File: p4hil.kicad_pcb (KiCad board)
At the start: 4 copper layers, 81.3 x 50.8 mm, 216 parts, among them J1 Conn_02x02_Odd_Even, J10 Conn_01x20, J11 Conn_01x20, J12 Conn_01x20, J13 USB_A_Stacked, J14 Conn_01x04, J15 Conn_01x20, J16 Conn_01x04, J17 Barrel_Jack_Switch, J18 Conn_02x05_Odd_Even, J19 HR871150C, J2 Conn_01x08, J3 USB_C_Receptacle_USB2.0_16P, J4 Conn_01x10, J5 Conn_01x20, J6 Conn_01x20, J7 Conn_01x20, J8 Conn_01x02, J9 Conn_01x06, SW1 SW_Push, SW2 SW_Push, U1 W25Q128JVS, U10 TLV62569DBV, U11 MT9700_SY6280, U3 TLV62569DBV, U4 IPGRI, U6 INA219AxD, U7 CH334F, U8 MT9700_SY6280, U9 MT9700_SY6280, Y1 40MHz(+-10 ppm) C501798, Y2 25Mhz 12pf, Y3 12MHz

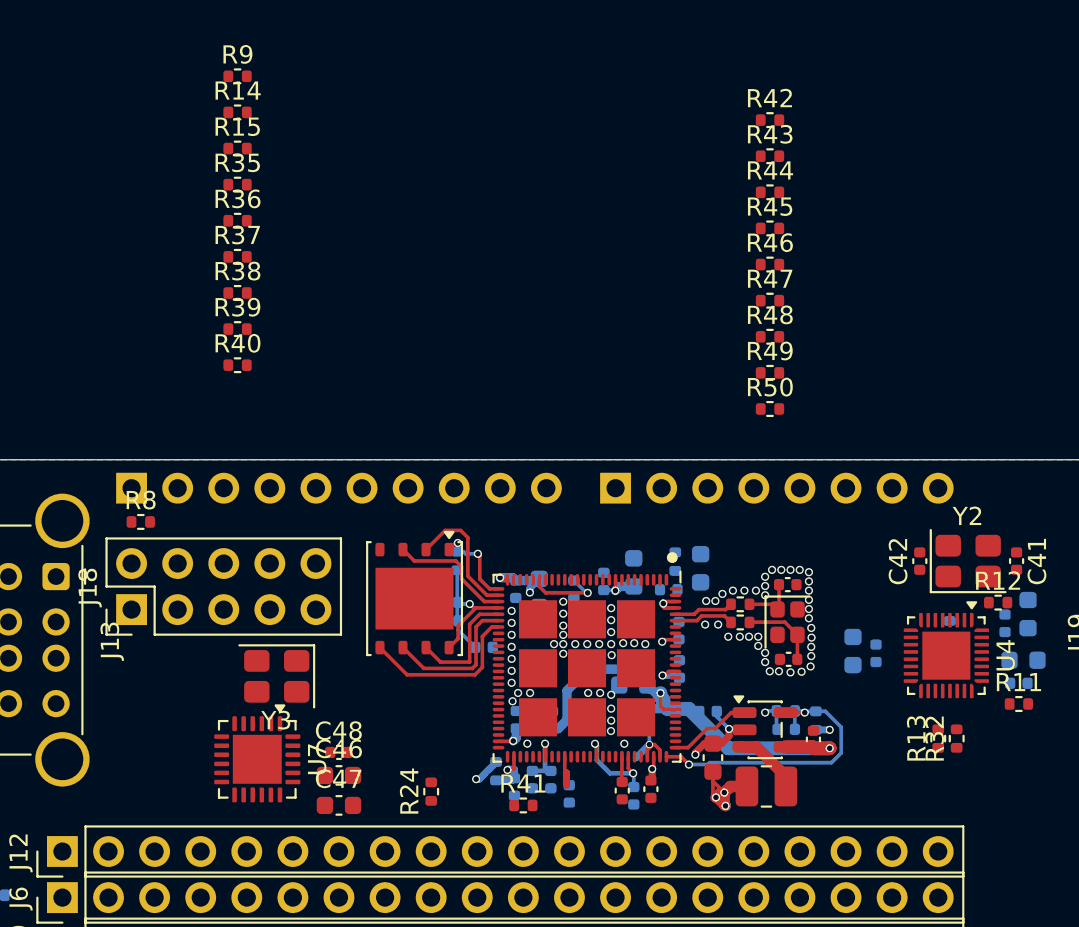
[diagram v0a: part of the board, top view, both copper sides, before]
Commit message: Drop T20'
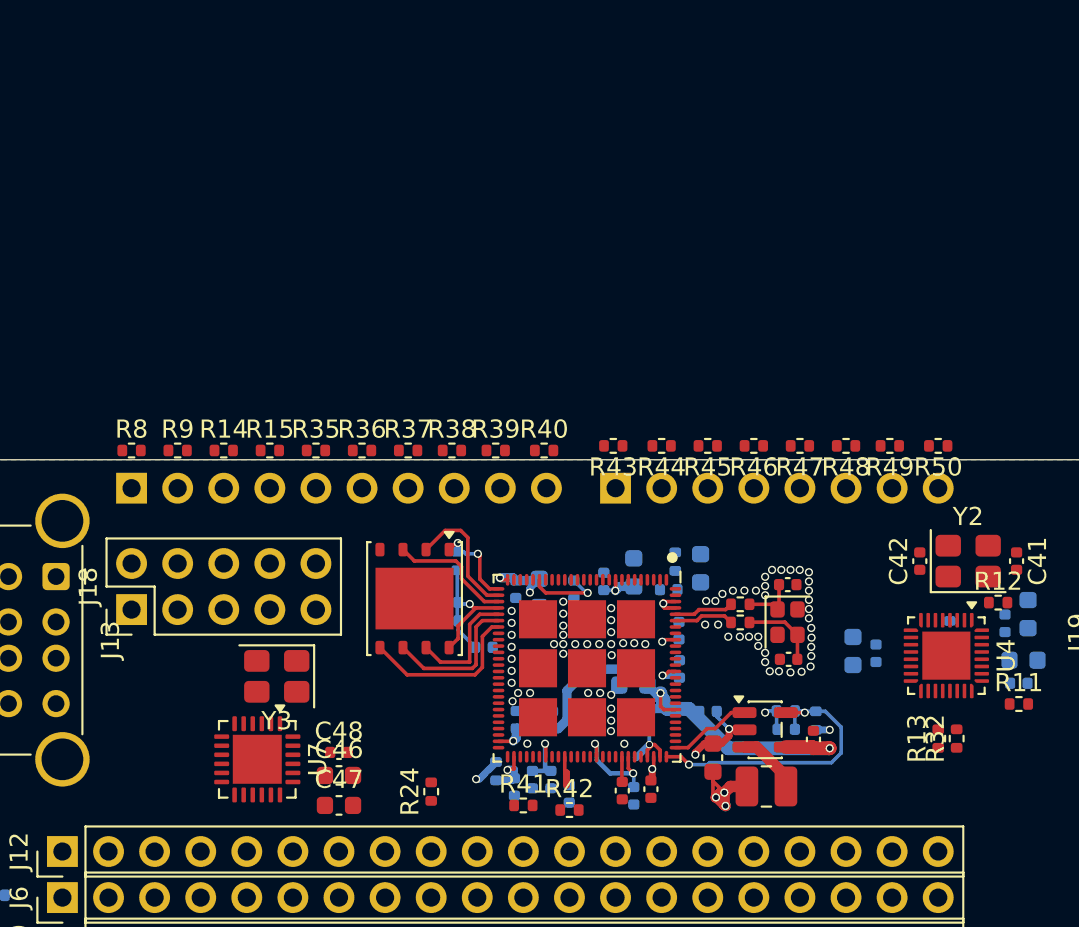
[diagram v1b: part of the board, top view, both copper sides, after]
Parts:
- moved R42 39.6 mm to (139.7, 92.7)
- moved R9 20.9 mm to (118.1, 72.9)
- moved R14 18.6 mm to (120.7, 72.9)
- moved R43 18.1 mm to (142.1, 72.6), turned to 180 degrees
- moved R40 17.5 mm to (138.3, 72.9)
- moved R15 16.7 mm to (123.2, 72.9)
- moved R39 15.7 mm to (135.6, 72.9)
- moved R35 15.3 mm to (125.7, 72.9)
- moved R44 15.2 mm to (144.8, 72.6), turned to 180 degrees
- moved R38 14.7 mm to (133.2, 72.9)
- moved R36 14.4 mm to (128.3, 72.9)
- moved R37 14.2 mm to (130.8, 72.9)
- moved R45 12.5 mm to (147.3, 72.6), turned to 180 degrees
- moved R46 10.0 mm to (149.9, 72.6), turned to 180 degrees
- moved R50 9.49 mm to (160.0, 72.6), turned to 180 degrees
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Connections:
- net /DeviceUnderTest/B1 renamed /B1
- net /DeviceUnderTest/B10 renamed /B10
- net /DeviceUnderTest/B11 renamed /B11
- net /DeviceUnderTest/B12 renamed /B12
- net /DeviceUnderTest/B13 renamed /B13
- net /DeviceUnderTest/B14 renamed /B14
- net /DeviceUnderTest/B15 renamed /B15
- net /DeviceUnderTest/B16 renamed /B16
- net /DeviceUnderTest/B17 renamed /B17
- net /DeviceUnderTest/B18 renamed /B18
- net /DeviceUnderTest/B19 renamed /B19
- net /DeviceUnderTest/B2 renamed /B2
- net /DeviceUnderTest/B20 renamed /B20
- net /DeviceUnderTest/B3 renamed /B3
- net /DeviceUnderTest/B4 renamed /B4
- net /DeviceUnderTest/B5 renamed /B5
- net /DeviceUnderTest/B6 renamed /B6
- net /DeviceUnderTest/B7 renamed /B7
- net /DeviceUnderTest/B8 renamed /B8
- net /DeviceUnderTest/B9 renamed /B9
- J10 pad 1: /DeviceUnderTest/T1 -> /DeviceUnderTest/T1i
- J10 pad 10: /DeviceUnderTest/T10 -> /DeviceUnderTest/T10i
- J10 pad 11: /DeviceUnderTest/ARDUINO_IOREF -> /DeviceUnderTest/T11i
- J10 pad 12: /DeviceUnderTest/ARDUINO_RESET -> /DeviceUnderTest/T12i
- J10 pad 13: /DeviceUnderTest/T13 -> /DeviceUnderTest/T13i
- J10 pad 14: /DeviceUnderTest/T14 -> /DeviceUnderTest/T14i
- J10 pad 15: /DeviceUnderTest/T15 -> /DeviceUnderTest/T15i
- J10 pad 16: /DeviceUnderTest/T16 -> /DeviceUnderTest/T16i
- J10 pad 17: /DeviceUnderTest/T17 -> /DeviceUnderTest/T17i
- J10 pad 18: /DeviceUnderTest/T18 -> /DeviceUnderTest/T18i
- J10 pad 19: /DeviceUnderTest/T19 -> /DeviceUnderTest/T19i
- J10 pad 2: /DeviceUnderTest/T2 -> /DeviceUnderTest/T2i
- J10 pad 20: /DeviceUnderTest/T20 -> /DeviceUnderTest/T20i
- J10 pad 3: /DeviceUnderTest/T3 -> /DeviceUnderTest/T3i
- J10 pad 4: /DeviceUnderTest/T4 -> /DeviceUnderTest/T4i
- J10 pad 5: /DeviceUnderTest/T5 -> /DeviceUnderTest/T5i
- J10 pad 6: /DeviceUnderTest/T6 -> /DeviceUnderTest/T6i
- J10 pad 7: /DeviceUnderTest/T7 -> /DeviceUnderTest/T7i
- J10 pad 8: /DeviceUnderTest/T8 -> /DeviceUnderTest/T8i
- J10 pad 9: /DeviceUnderTest/T9 -> /DeviceUnderTest/T9i
- J11 pad 1: /DeviceUnderTest/T1 -> /DeviceUnderTest/T1i
- J11 pad 10: /DeviceUnderTest/T10 -> /DeviceUnderTest/T10i
- J11 pad 11: /DeviceUnderTest/ARDUINO_IOREF -> /DeviceUnderTest/T11i
- J11 pad 12: /DeviceUnderTest/ARDUINO_RESET -> /DeviceUnderTest/T12i
- J11 pad 13: /DeviceUnderTest/T13 -> /DeviceUnderTest/T13i
- J11 pad 14: /DeviceUnderTest/T14 -> /DeviceUnderTest/T14i
- J11 pad 15: /DeviceUnderTest/T15 -> /DeviceUnderTest/T15i
- J11 pad 16: /DeviceUnderTest/T16 -> /DeviceUnderTest/T16i
- J11 pad 17: /DeviceUnderTest/T17 -> /DeviceUnderTest/T17i
- J11 pad 18: /DeviceUnderTest/T18 -> /DeviceUnderTest/T18i
- J11 pad 19: /DeviceUnderTest/T19 -> /DeviceUnderTest/T19i
- J11 pad 2: /DeviceUnderTest/T2 -> /DeviceUnderTest/T2i
- J11 pad 20: /DeviceUnderTest/T20 -> /DeviceUnderTest/T20i
- J11 pad 3: /DeviceUnderTest/T3 -> /DeviceUnderTest/T3i
- J11 pad 4: /DeviceUnderTest/T4 -> /DeviceUnderTest/T4i
- J11 pad 5: /DeviceUnderTest/T5 -> /DeviceUnderTest/T5i
- J11 pad 6: /DeviceUnderTest/T6 -> /DeviceUnderTest/T6i
- J11 pad 7: /DeviceUnderTest/T7 -> /DeviceUnderTest/T7i
- J11 pad 8: /DeviceUnderTest/T8 -> /DeviceUnderTest/T8i
- J11 pad 9: /DeviceUnderTest/T9 -> /DeviceUnderTest/T9i
- J12 pad 1: /DeviceUnderTest/T1 -> /DeviceUnderTest/T1i
- J12 pad 10: /DeviceUnderTest/T10 -> /DeviceUnderTest/T10i
- J12 pad 11: /DeviceUnderTest/ARDUINO_IOREF -> /DeviceUnderTest/T11i
- J12 pad 12: /DeviceUnderTest/ARDUINO_RESET -> /DeviceUnderTest/T12i
- J12 pad 13: /DeviceUnderTest/T13 -> /DeviceUnderTest/T13i
- J12 pad 14: /DeviceUnderTest/T14 -> /DeviceUnderTest/T14i
- J12 pad 15: /DeviceUnderTest/T15 -> /DeviceUnderTest/T15i
- J12 pad 16: /DeviceUnderTest/T16 -> /DeviceUnderTest/T16i
- J12 pad 17: /DeviceUnderTest/T17 -> /DeviceUnderTest/T17i
- J12 pad 18: /DeviceUnderTest/T18 -> /DeviceUnderTest/T18i
- J12 pad 19: /DeviceUnderTest/T19 -> /DeviceUnderTest/T19i
- J12 pad 2: /DeviceUnderTest/T2 -> /DeviceUnderTest/T2i
- J12 pad 20: /DeviceUnderTest/T20 -> /DeviceUnderTest/T20i
- J12 pad 3: /DeviceUnderTest/T3 -> /DeviceUnderTest/T3i
- J12 pad 4: /DeviceUnderTest/T4 -> /DeviceUnderTest/T4i
- J12 pad 5: /DeviceUnderTest/T5 -> /DeviceUnderTest/T5i
- J12 pad 6: /DeviceUnderTest/T6 -> /DeviceUnderTest/T6i
- J12 pad 7: /DeviceUnderTest/T7 -> /DeviceUnderTest/T7i
- J12 pad 8: /DeviceUnderTest/T8 -> /DeviceUnderTest/T8i
- J12 pad 9: /DeviceUnderTest/T9 -> /DeviceUnderTest/T9i
- J15 pad 1: /DeviceUnderTest/T1 -> /DeviceUnderTest/T1i
- J15 pad 10: /DeviceUnderTest/T10 -> /DeviceUnderTest/T10i
- J15 pad 11: /DeviceUnderTest/ARDUINO_IOREF -> /DeviceUnderTest/T11i
- J15 pad 12: /DeviceUnderTest/ARDUINO_RESET -> /DeviceUnderTest/T12i
- J15 pad 13: /DeviceUnderTest/T13 -> /DeviceUnderTest/T13i
- J15 pad 14: /DeviceUnderTest/T14 -> /DeviceUnderTest/T14i
- J15 pad 15: /DeviceUnderTest/T15 -> /DeviceUnderTest/T15i
- J15 pad 16: /DeviceUnderTest/T16 -> /DeviceUnderTest/T16i
- J15 pad 17: /DeviceUnderTest/T17 -> /DeviceUnderTest/T17i
- J15 pad 18: /DeviceUnderTest/T18 -> /DeviceUnderTest/T18i
- J15 pad 19: /DeviceUnderTest/T19 -> /DeviceUnderTest/T19i
- J15 pad 2: /DeviceUnderTest/T2 -> /DeviceUnderTest/T2i
- J15 pad 20: /DeviceUnderTest/T20 -> /DeviceUnderTest/T20i
- J15 pad 3: /DeviceUnderTest/T3 -> /DeviceUnderTest/T3i
- J15 pad 4: /DeviceUnderTest/T4 -> /DeviceUnderTest/T4i
- J15 pad 5: /DeviceUnderTest/T5 -> /DeviceUnderTest/T5i
- J15 pad 6: /DeviceUnderTest/T6 -> /DeviceUnderTest/T6i
- J15 pad 7: /DeviceUnderTest/T7 -> /DeviceUnderTest/T7i
- J15 pad 8: /DeviceUnderTest/T8 -> /DeviceUnderTest/T8i
- J15 pad 9: /DeviceUnderTest/T9 -> /DeviceUnderTest/T9i
- J2 pad 1: /DeviceUnderTest/T13 -> /DeviceUnderTest/T13i
- J2 pad 2: /DeviceUnderTest/T14 -> /DeviceUnderTest/T14i
- J2 pad 3: /DeviceUnderTest/T15 -> /DeviceUnderTest/T15i
- J2 pad 4: /DeviceUnderTest/T16 -> /DeviceUnderTest/T16i
- J2 pad 5: /DeviceUnderTest/T17 -> /DeviceUnderTest/T17i
- J2 pad 6: /DeviceUnderTest/T18 -> /DeviceUnderTest/T18i
- J2 pad 7: /DeviceUnderTest/T19 -> /DeviceUnderTest/T19i
- J2 pad 8: /DeviceUnderTest/T20 -> /DeviceUnderTest/T20i
- J4 pad 1: /DeviceUnderTest/T1 -> /DeviceUnderTest/T1i
- J4 pad 10: /DeviceUnderTest/T10 -> /DeviceUnderTest/T10i
- J4 pad 2: /DeviceUnderTest/T2 -> /DeviceUnderTest/T2i
- J4 pad 3: /DeviceUnderTest/T3 -> /DeviceUnderTest/T3i
- J4 pad 4: /DeviceUnderTest/T4 -> /DeviceUnderTest/T4i
- J4 pad 5: /DeviceUnderTest/T5 -> /DeviceUnderTest/T5i
- J4 pad 6: /DeviceUnderTest/T6 -> /DeviceUnderTest/T6i
- J4 pad 7: /DeviceUnderTest/T7 -> /DeviceUnderTest/T7i
- J4 pad 8: /DeviceUnderTest/T8 -> /DeviceUnderTest/T8i
- J4 pad 9: /DeviceUnderTest/T9 -> /DeviceUnderTest/T9i
- J6 pad 1: /DeviceUnderTest/T1 -> /DeviceUnderTest/T1i
- J6 pad 10: /DeviceUnderTest/T10 -> /DeviceUnderTest/T10i
- J6 pad 11: /DeviceUnderTest/ARDUINO_IOREF -> /DeviceUnderTest/T11i
- J6 pad 12: /DeviceUnderTest/ARDUINO_RESET -> /DeviceUnderTest/T12i
- J6 pad 13: /DeviceUnderTest/T13 -> /DeviceUnderTest/T13i
- J6 pad 14: /DeviceUnderTest/T14 -> /DeviceUnderTest/T14i
- J6 pad 15: /DeviceUnderTest/T15 -> /DeviceUnderTest/T15i
- J6 pad 16: /DeviceUnderTest/T16 -> /DeviceUnderTest/T16i
- J6 pad 17: /DeviceUnderTest/T17 -> /DeviceUnderTest/T17i
- J6 pad 18: /DeviceUnderTest/T18 -> /DeviceUnderTest/T18i
- J6 pad 19: /DeviceUnderTest/T19 -> /DeviceUnderTest/T19i
- J6 pad 2: /DeviceUnderTest/T2 -> /DeviceUnderTest/T2i
- J6 pad 20: /DeviceUnderTest/T20 -> /DeviceUnderTest/T20i
- J6 pad 3: /DeviceUnderTest/T3 -> /DeviceUnderTest/T3i
- J6 pad 4: /DeviceUnderTest/T4 -> /DeviceUnderTest/T4i
- J6 pad 5: /DeviceUnderTest/T5 -> /DeviceUnderTest/T5i
- J6 pad 6: /DeviceUnderTest/T6 -> /DeviceUnderTest/T6i
- J6 pad 7: /DeviceUnderTest/T7 -> /DeviceUnderTest/T7i
- J6 pad 8: /DeviceUnderTest/T8 -> /DeviceUnderTest/T8i
- J6 pad 9: /DeviceUnderTest/T9 -> /DeviceUnderTest/T9i
- J7 pad 1: /DeviceUnderTest/T1 -> /DeviceUnderTest/T1i
- J7 pad 10: /DeviceUnderTest/T10 -> /DeviceUnderTest/T10i
- J7 pad 11: /DeviceUnderTest/ARDUINO_IOREF -> /DeviceUnderTest/T11i
- J7 pad 12: /DeviceUnderTest/ARDUINO_RESET -> /DeviceUnderTest/T12i
- J7 pad 13: /DeviceUnderTest/T13 -> /DeviceUnderTest/T13i
- J7 pad 14: /DeviceUnderTest/T14 -> /DeviceUnderTest/T14i
- J7 pad 15: /DeviceUnderTest/T15 -> /DeviceUnderTest/T15i
- J7 pad 16: /DeviceUnderTest/T16 -> /DeviceUnderTest/T16i
- J7 pad 17: /DeviceUnderTest/T17 -> /DeviceUnderTest/T17i
- J7 pad 18: /DeviceUnderTest/T18 -> /DeviceUnderTest/T18i
- J7 pad 19: /DeviceUnderTest/T19 -> /DeviceUnderTest/T19i
- J7 pad 2: /DeviceUnderTest/T2 -> /DeviceUnderTest/T2i
- J7 pad 20: /DeviceUnderTest/T20 -> /DeviceUnderTest/T20i
- J7 pad 3: /DeviceUnderTest/T3 -> /DeviceUnderTest/T3i
- J7 pad 4: /DeviceUnderTest/T4 -> /DeviceUnderTest/T4i
- J7 pad 5: /DeviceUnderTest/T5 -> /DeviceUnderTest/T5i
- J7 pad 6: /DeviceUnderTest/T6 -> /DeviceUnderTest/T6i
- J7 pad 7: /DeviceUnderTest/T7 -> /DeviceUnderTest/T7i
- J7 pad 8: /DeviceUnderTest/T8 -> /DeviceUnderTest/T8i
- J7 pad 9: /DeviceUnderTest/T9 -> /DeviceUnderTest/T9i
- J8 pad 1: /DeviceUnderTest/ARDUINO_IOREF -> /T11
- J8 pad 2: /DeviceUnderTest/ARDUINO_RESET -> /T12
- R14 pad 1: /DeviceUnderTest/T3 -> /DeviceUnderTest/T3i
- R14 pad 2: /DeviceUnderTest/T3 -> /T3
- R15 pad 1: /DeviceUnderTest/T4 -> /DeviceUnderTest/T4i
- R15 pad 2: /DeviceUnderTest/T4 -> /T4
- R32 pad 2: /Ethernet/MDC -> /MDC
- R35 pad 1: /DeviceUnderTest/T5 -> /DeviceUnderTest/T5i
- R35 pad 2: /DeviceUnderTest/T5 -> /T5
- R36 pad 1: /DeviceUnderTest/T6 -> /DeviceUnderTest/T6i
- R36 pad 2: /DeviceUnderTest/T6 -> /T6
- R37 pad 1: /DeviceUnderTest/T7 -> /DeviceUnderTest/T7i
- R37 pad 2: /DeviceUnderTest/T7 -> /T7
- R38 pad 1: /DeviceUnderTest/T8 -> /DeviceUnderTest/T8i
- R38 pad 2: /DeviceUnderTest/T8 -> /T8
- R39 pad 1: /DeviceUnderTest/T9 -> /DeviceUnderTest/T9i
- R39 pad 2: /DeviceUnderTest/T9 -> /T9
- R40 pad 1: /DeviceUnderTest/T10 -> /DeviceUnderTest/T10i
- R40 pad 2: /DeviceUnderTest/T10 -> /T10
- R41 pad 1: /DeviceUnderTest/ARDUINO_IOREF -> /DeviceUnderTest/T11i
- R41 pad 2: /DeviceUnderTest/ARDUINO_IOREF -> /T11
- R42 pad 1: /DeviceUnderTest/ARDUINO_RESET -> /DeviceUnderTest/T12i
- R42 pad 2: /DeviceUnderTest/ARDUINO_RESET -> /T12
- R43 pad 1: /DeviceUnderTest/T13 -> /DeviceUnderTest/T13i
- R43 pad 2: /DeviceUnderTest/T13 -> /T13
- R44 pad 1: /DeviceUnderTest/T14 -> /DeviceUnderTest/T14i
- R44 pad 2: /DeviceUnderTest/T14 -> /T14
- R45 pad 1: /DeviceUnderTest/T15 -> /DeviceUnderTest/T15i
- R45 pad 2: /DeviceUnderTest/T15 -> /T15
- R46 pad 1: /DeviceUnderTest/T16 -> /DeviceUnderTest/T16i
- R46 pad 2: /DeviceUnderTest/T16 -> /T16
- R47 pad 1: /DeviceUnderTest/T17 -> /DeviceUnderTest/T17i
- R47 pad 2: /DeviceUnderTest/T17 -> /T17
- R48 pad 1: /DeviceUnderTest/T18 -> /DeviceUnderTest/T18i
- R48 pad 2: /DeviceUnderTest/T18 -> /T18
- R49 pad 1: /DeviceUnderTest/T19 -> /DeviceUnderTest/T19i
- R49 pad 2: /DeviceUnderTest/T19 -> /T19
- R50 pad 1: /DeviceUnderTest/T20 -> /DeviceUnderTest/T20i
- R50 pad 2: /DeviceUnderTest/T20 -> /T20
- R74 pad 2: /DeviceUnderTest/T1 -> /DeviceUnderTest/T1i
- R75 pad 2: /DeviceUnderTest/T2 -> /DeviceUnderTest/T2i
- R76 pad 2: /DeviceUnderTest/T3 -> /DeviceUnderTest/T3i
- R77 pad 2: /DeviceUnderTest/T4 -> /DeviceUnderTest/T4i
- R78 pad 2: /DeviceUnderTest/T5 -> /DeviceUnderTest/T5i
- R79 pad 2: /DeviceUnderTest/T6 -> /DeviceUnderTest/T6i
- R8 pad 1: /DeviceUnderTest/T1 -> /DeviceUnderTest/T1i
- R8 pad 2: /DeviceUnderTest/T1 -> /T1
- R80 pad 2: /DeviceUnderTest/T7 -> /DeviceUnderTest/T7i
- R81 pad 2: /DeviceUnderTest/T8 -> /DeviceUnderTest/T8i
- R82 pad 2: /DeviceUnderTest/T9 -> /DeviceUnderTest/T9i
- R83 pad 2: /DeviceUnderTest/T10 -> /DeviceUnderTest/T10i
- R84 pad 2: /DeviceUnderTest/ARDUINO_IOREF -> /DeviceUnderTest/T11i
- R85 pad 2: /DeviceUnderTest/ARDUINO_RESET -> /DeviceUnderTest/T12i
- R86 pad 2: /DeviceUnderTest/T13 -> /DeviceUnderTest/T13i
- R87 pad 2: /DeviceUnderTest/T14 -> /DeviceUnderTest/T14i
- R88 pad 2: /DeviceUnderTest/T15 -> /DeviceUnderTest/T15i
- R89 pad 2: /DeviceUnderTest/T16 -> /DeviceUnderTest/T16i
- R9 pad 1: /DeviceUnderTest/T2 -> /DeviceUnderTest/T2i
- R9 pad 2: /DeviceUnderTest/T2 -> /T2
- R90 pad 2: /DeviceUnderTest/T17 -> /DeviceUnderTest/T17i
- R91 pad 2: /DeviceUnderTest/T18 -> /DeviceUnderTest/T18i
- R92 pad 2: /DeviceUnderTest/T19 -> /DeviceUnderTest/T19i
- R93 pad 2: /DeviceUnderTest/T20 -> /DeviceUnderTest/T20i
- U2 pad 1: /P4/GPIO1/ADC -> /T14
- U2 pad 10: /P4/GPIO9/ADC -> /T6
- U2 pad 11: /P4/GPIO10/ADC -> /T5
- U2 pad 12: /P4/GPIO11/ADC -> /T4
- U2 pad 13: /P4/GPIO12/ADC -> /T3
- U2 pad 14: /P4/GPIO13/ADC -> /T2
- U2 pad 15: /P4/GPIO14/ADC -> /T1
- U2 pad 2: /P4/GPIO2/ADC -> /T13
- U2 pad 3: /P4/GPIO3/ADC -> /T12
- U2 pad 4: /P4/GPIO4/ADC -> /T11
- U2 pad 5: /P4/GPIO5/ADC -> /T10
- U2 pad 6: /P4/GPIO6/ADC -> /T9
- U2 pad 7: /P4/GPIO7/ADC -> /T8
- U2 pad 8: /P4/GPIO8/ADC -> /T7
- U2 pad 84: /P4/GPIO43 -> /MDIO
- U2 pad 90: /P4/GPIO48 -> /MDC
- U2 pad 92: /P4/GPIO49/ADC -> /T20
- U2 pad 93: /P4/GPIO50/ADC -> /T19
- U2 pad 94: /P4/GPIO51/ADC -> /T18
- U2 pad 95: /P4/GPIO52/ADC -> /T17
- U2 pad 97: /P4/GPIO53/ADC -> /T16
- U2 pad 98: /P4/GPIO54/ADC -> /T15
- U4 pad 22: /Ethernet/MDC -> /MDC
- U4 pad 23: /Ethernet/MDIO -> /MDIO
